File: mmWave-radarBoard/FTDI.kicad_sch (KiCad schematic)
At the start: 42 parts, among them U301 FT4232H, U302 93LCxxB, Y301 12MHz

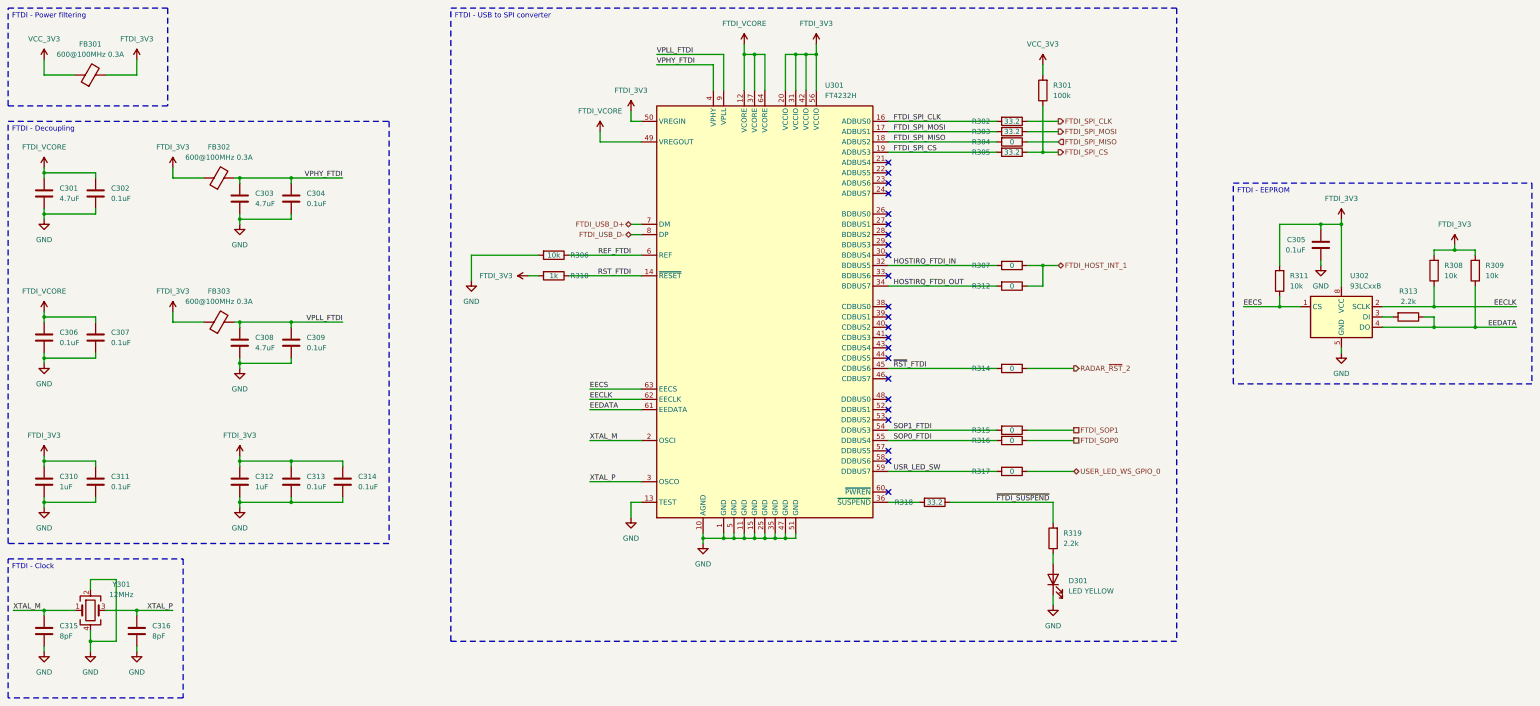
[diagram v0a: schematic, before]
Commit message: Updated radar PCB and schematic
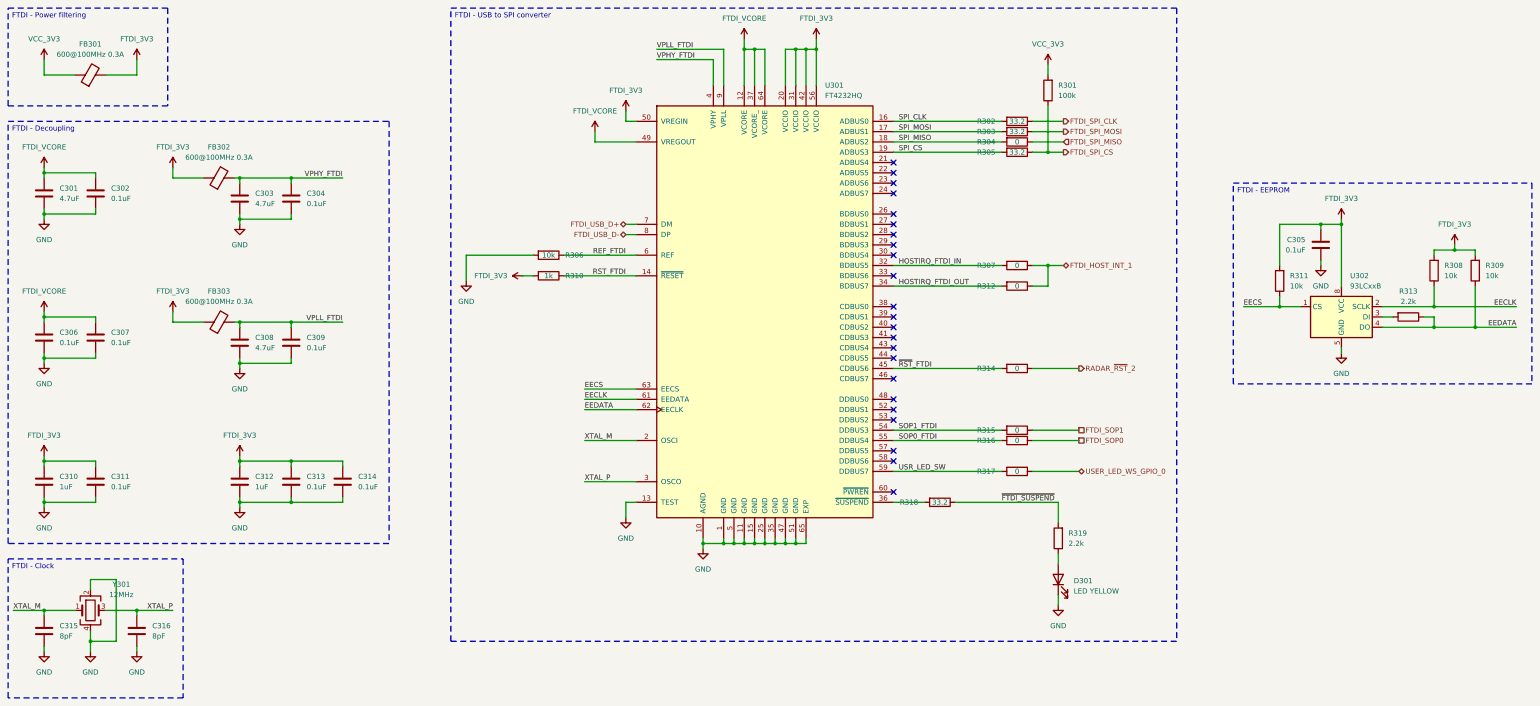
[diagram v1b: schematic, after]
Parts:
- removed U301: FT4232H, Package_QFP:LQFP-64_10x10mm_P0.5mm, symbol Interface_USB:FT4232H
- added U301: FT4232HQ, FT4232HQ:QFN50P900X900X105-65N, symbol FT4232HQ:FT4232HQ
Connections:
- net EECLK: now also U301.61 (EEDATA)
- net EECS: now also U301.63 (EECS)
- net EEDATA: now also U301.62 (EECLK)
- net FTDI_3V3: now also U301.20 (VCCIO), U301.31 (VCCIO), U301.42 (VCCIO), U301.50 (VREGIN), U301.56 (VCCIO)
- net FTDI_SPI_CLK: no longer R302.2
- net FTDI_SPI_CS: no longer R305.2
- net FTDI_SPI_MISO: no longer R304.2
- net FTDI_SPI_MOSI: no longer R303.2
- net FTDI_USB_D+: now also U301.7 (DM)
- net FTDI_USB_D-: now also U301.8 (DP)
- net FTDI_VCORE: now also U301.12 (VCORE), U301.37 (VCORE_), U301.49 (VREGOUT), U301.64 (VCORE)
- net GND: now also U301.1 (GND), U301.10 (AGND), U301.11 (GND), U301.13 (TEST), U301.15 (GND), U301.25 (GND), U301.35 (GND), U301.47 (GND), U301.5 (GND), U301.51 (GND), U301.65 (EXP)
- net HOSTIRQ_FTDI_IN: now also U301.32 (BDBUS5)
- net HOSTIRQ_FTDI_OUT: now also U301.34 (BDBUS7)
- net REF_FTDI: now also U301.6 (REF)
- net RST_FTDI: now also U301.14 (~{RESET})
- net SOP0_FTDI: now also U301.55 (DDBUS4)
- net SOP1_FTDI: now also U301.54 (DDBUS3)
- net USR_LED_SW: now also U301.59 (DDBUS7)
- net VPHY_FTDI: now also U301.4 (VPHY)
- net VPLL_FTDI: now also U301.9 (VPLL)
- net XTAL_M: now also U301.2 (OSCI)
- net XTAL_P: now also U301.3 (OSCO)
- net ~{RST}_FTDI: now also U301.45 (CDBUS6)
- net at R318.2: now also U301.36 (~{SUSPEND})
- new net SPI_CLK: R302.2, U301.16 (ADBUS0)
- new net SPI_CS: R305.2, U301.19 (ADBUS3)
- new net SPI_MISO: R304.2, U301.18 (ADBUS2)
- new net SPI_MOSI: R303.2, U301.17 (ADBUS1)
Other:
- moved on the sheet: D301, R301, R302, R303, R304, R305, R306, R307, R310, R312, R314, R315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
